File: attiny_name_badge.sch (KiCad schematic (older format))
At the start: 16 parts, among them U1 ATtiny841-SSU

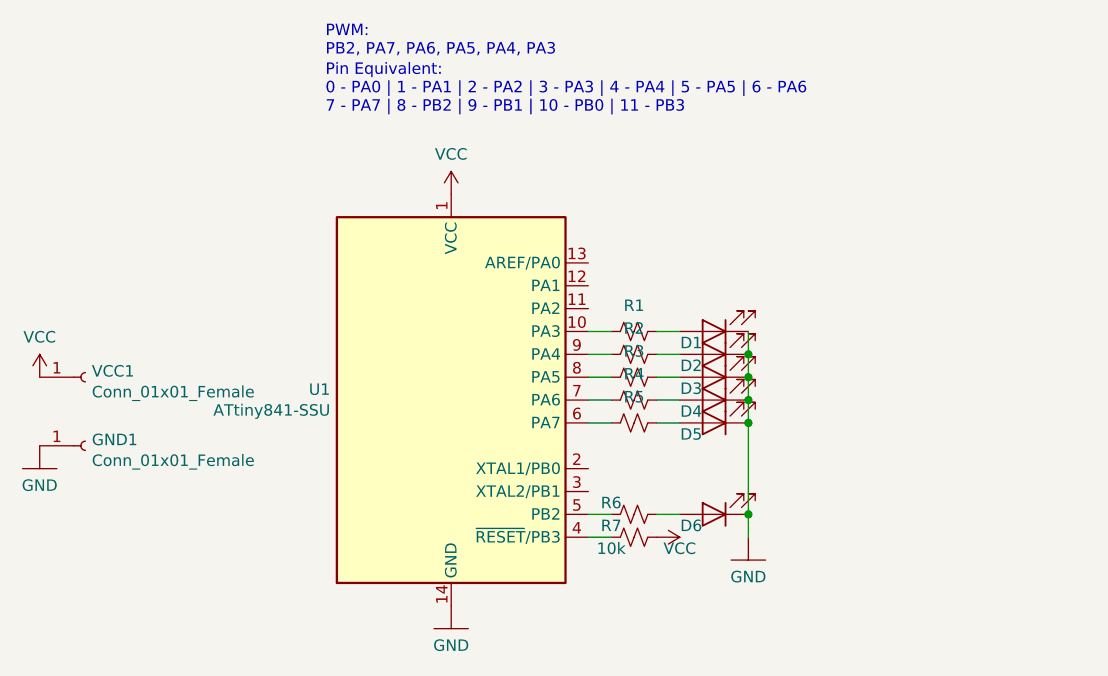
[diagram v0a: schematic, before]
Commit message: working circuit
need name/finishing touches
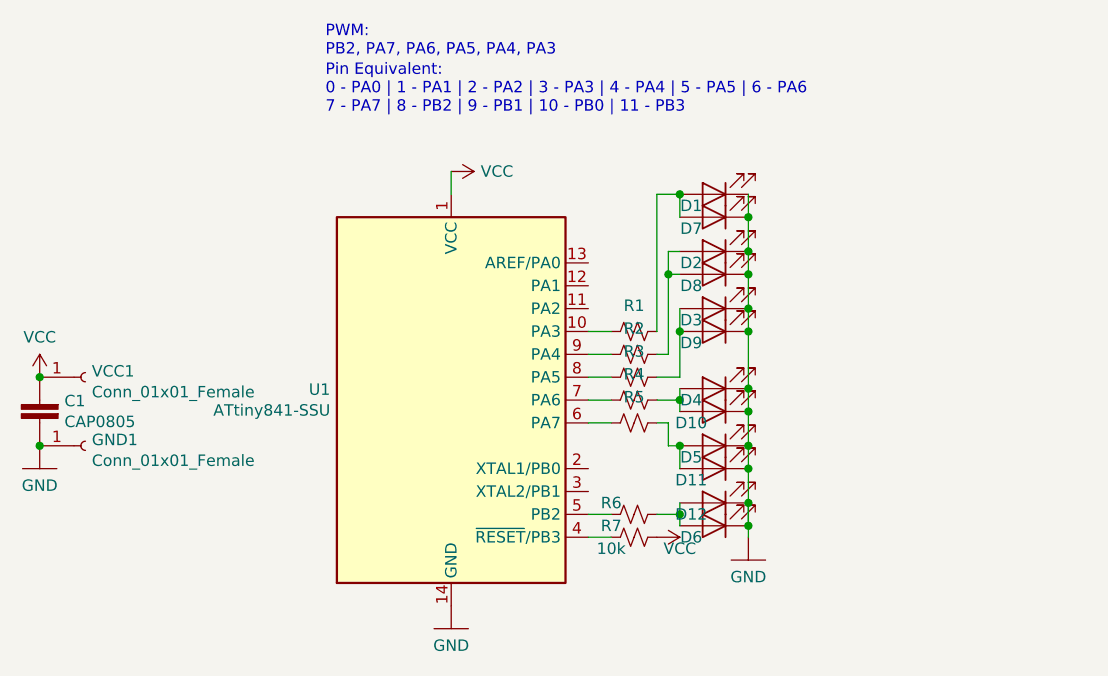
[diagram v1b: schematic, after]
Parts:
- added C1: CAP0805, Capacitor_SMD:C_0805_2012Metric_Pad1.15x1.40mm_HandSolder, symbol SparkFun-Capacitors:CAP0805
- added D10, D11, D12, D7, D8, D9: LED, LED_SMD:LED_0805_2012Metric_Pad1.15x1.40mm_HandSolder, symbol Device:LED
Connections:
- net GND: now also C1.1, D10.1 (K), D11.1 (K), D12.1 (K), D7.1 (K), D8.1 (K), D9.1 (K)
- net VCC: now also C1.2
- net at D1.2 (A), R1.1: now also D7.2 (A)
- net at D2.2 (A), R2.1: now also D8.2 (A)
- net at D3.2 (A), R3.1: now also D9.2 (A)
- net at D4.2 (A), R4.1: now also D10.2 (A)
- net at D5.2 (A), R5.1: now also D11.2 (A)
- net at D6.2 (A), R6.1: now also D12.2 (A)
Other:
- moved on the sheet: D1, D2, D3, D4, D5, D6

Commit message: working board
cut 'er out!
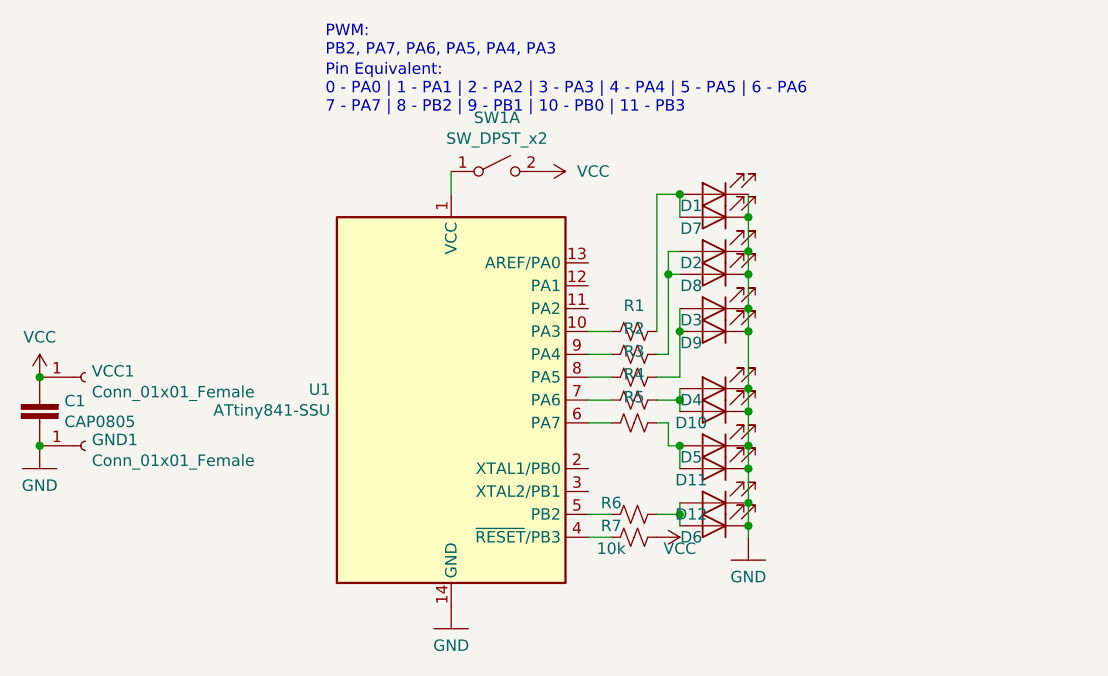
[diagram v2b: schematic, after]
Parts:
- added SW1: SW_DPST_x2, Button_Switch_THT:SW_PUSH_6mm_H5mm, symbol Switch:SW_DPST_x2
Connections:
- net VCC: now also SW1.2 (B); no longer U1.1 (VCC)
- new net: SW1.1 (A), U1.1 (VCC)
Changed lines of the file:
@@
 L SparkFun-Aesthetics:VCC #SUPPLY0101
 U 1 1 5D696DEA
-P 6100 2300
-F 0 "#SUPPLY0101" H 6100 2300 50  0001 L BNN
-F 1 "VCC" V 6100 2429 50  0000 L CNN
-F 2 "" H 6100 2300 50  0001 C CNN
-F 3 "" H 6100 2300 50  0001 C CNN
-	1    6100 2300
+P 6500 2300
+F 0 "#SUPPLY0101" H 6500 2300 50  0001 L BNN
+F 1 "VCC" V 6500 2450 50  0000 L CNN
+F 2 "" H 6500 2300 50  0001 C CNN
+F 3 "" H 6500 2300 50  0001 C CNN
+	1    6500 2300
 	0    1    1    0
 $EndComp
@@
 	7400 3850 7400 3750
 Connection ~ 7400 3750
-Wire Wire Line
-	7400 3750 7400 3850
 Connection ~ 4300 3500
 Connection ~ 4300 3200
+$Comp
+L Switch:SW_DPST_x2 SW1
+U 1 1 5D7BF4E8
+P 6300 2300
+F 0 "SW1" H 6300 2535 50  0000 C CNN
+F 1 "SW_DPST_x2" H 6300 2444 50  0000 C CNN
+F 2 "Button_Switch_THT:SW_PUSH_6mm_H5mm" H 6300 2300 50  0001 C CNN
+F 3 "~" H 6300 2300 50  0001 C CNN
+	1    6300 2300
+	1    0    0    -1
+$EndComp
 $EndSCHEMATC
